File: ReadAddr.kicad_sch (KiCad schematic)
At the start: 8 parts, among them U501 74HC163, U502 74HC163, U503 74HC163, U504 74HC163

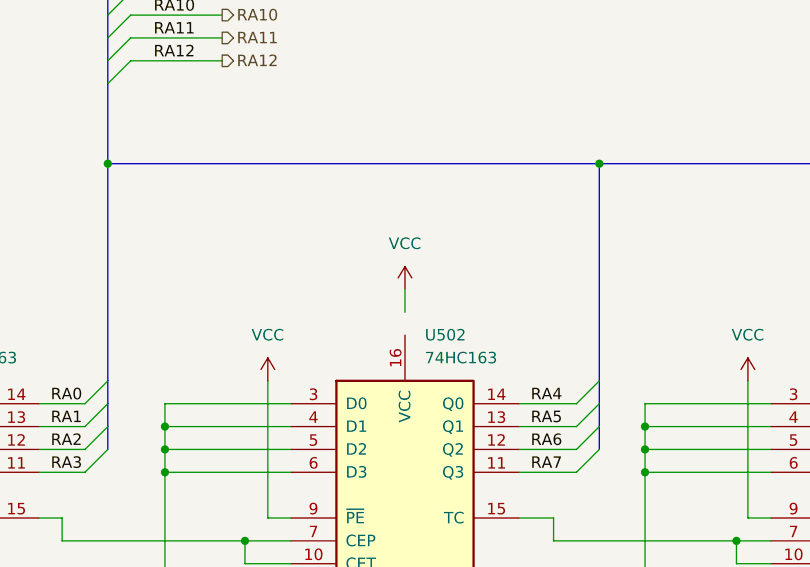
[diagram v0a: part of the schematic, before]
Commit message: start working on VRAM/read logic
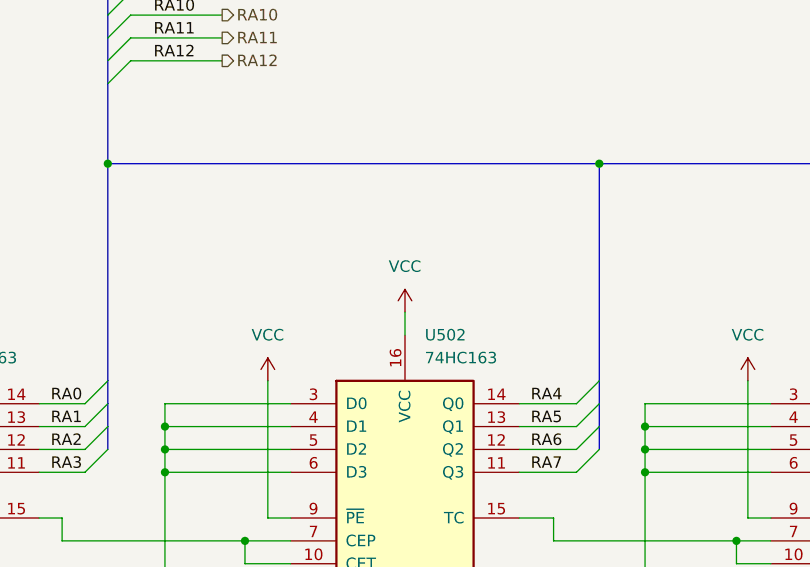
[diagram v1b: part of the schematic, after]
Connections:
- net VCC: now also U502.16 (VCC)
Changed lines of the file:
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@@
 	(wire
 		(pts
-			(xy 110.49 96.52) (xy 110.49 99.06)
+			(xy 110.49 99.06) (xy 110.49 101.6)
 		)
 		(stroke
@@
 	(symbol
 		(lib_id "power:VCC")
-		(at 110.49 96.52 0)
+		(at 110.49 99.06 0)
 		(unit 1)
 		(exclude_from_sim no)
@@
 		(fields_autoplaced yes)
 		(property "Reference" "#PWR048"
-			(at 110.49 100.33 0)
+			(at 110.49 102.87 0)
 			(effects
 				(font
@@
 		)
 		(property "Value" "VCC"
-			(at 110.49 91.44 0)
+			(at 110.49 93.98 0)
 			(effects
 				(font
@@
 		)
 		(property "Footprint" ""
-			(at 110.49 96.52 0)
+			(at 110.49 99.06 0)
 			(effects
 				(font
@@
 		)
 		(property "Datasheet" ""
-			(at 110.49 96.52 0)
+			(at 110.49 99.06 0)
 			(effects
 				(font
@@
 		)
 		(property "Description" "Power symbol creates a global label with name \"VCC\""
-			(at 110.49 96.52 0)
-			(effects
-				(font
+			(at 110.49 99.06 0)
+			(effects
+				(font
